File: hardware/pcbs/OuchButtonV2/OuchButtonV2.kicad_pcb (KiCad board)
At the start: 4 copper layers, 78 parts, among them J1 USB_C_Receptacle_USB2.0_14P, J3 Conn_01x01_Pin, Q1 AO3423 P-Chanel, U1 ESP32-C6-MINI-1/U, U2 RT9080-33GJ5, U3 MCP73831-2-OT, U4 MPU-6050, U5 DS1307Z+, U6 AT42QT1010-TSHR, U7 TS3A24159DGS, U8 AFE4404YZPT, U9 WE-TVS-82400102, Y1 32.768 kHz

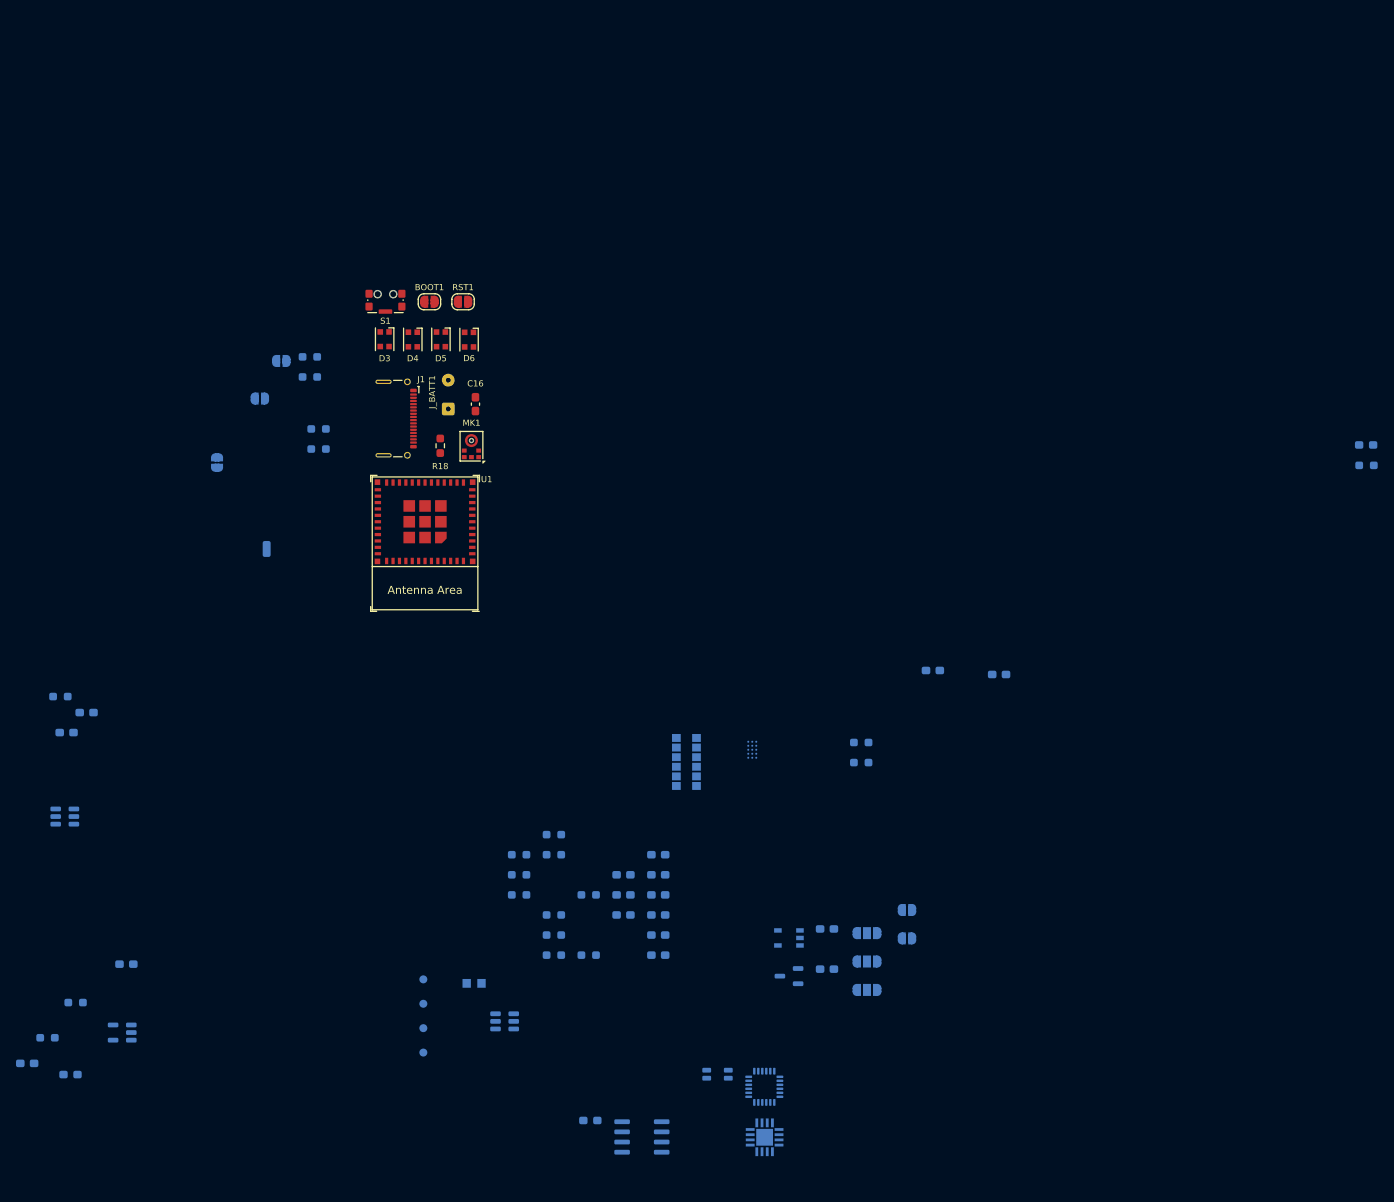
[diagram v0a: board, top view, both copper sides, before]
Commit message: Half done pcb
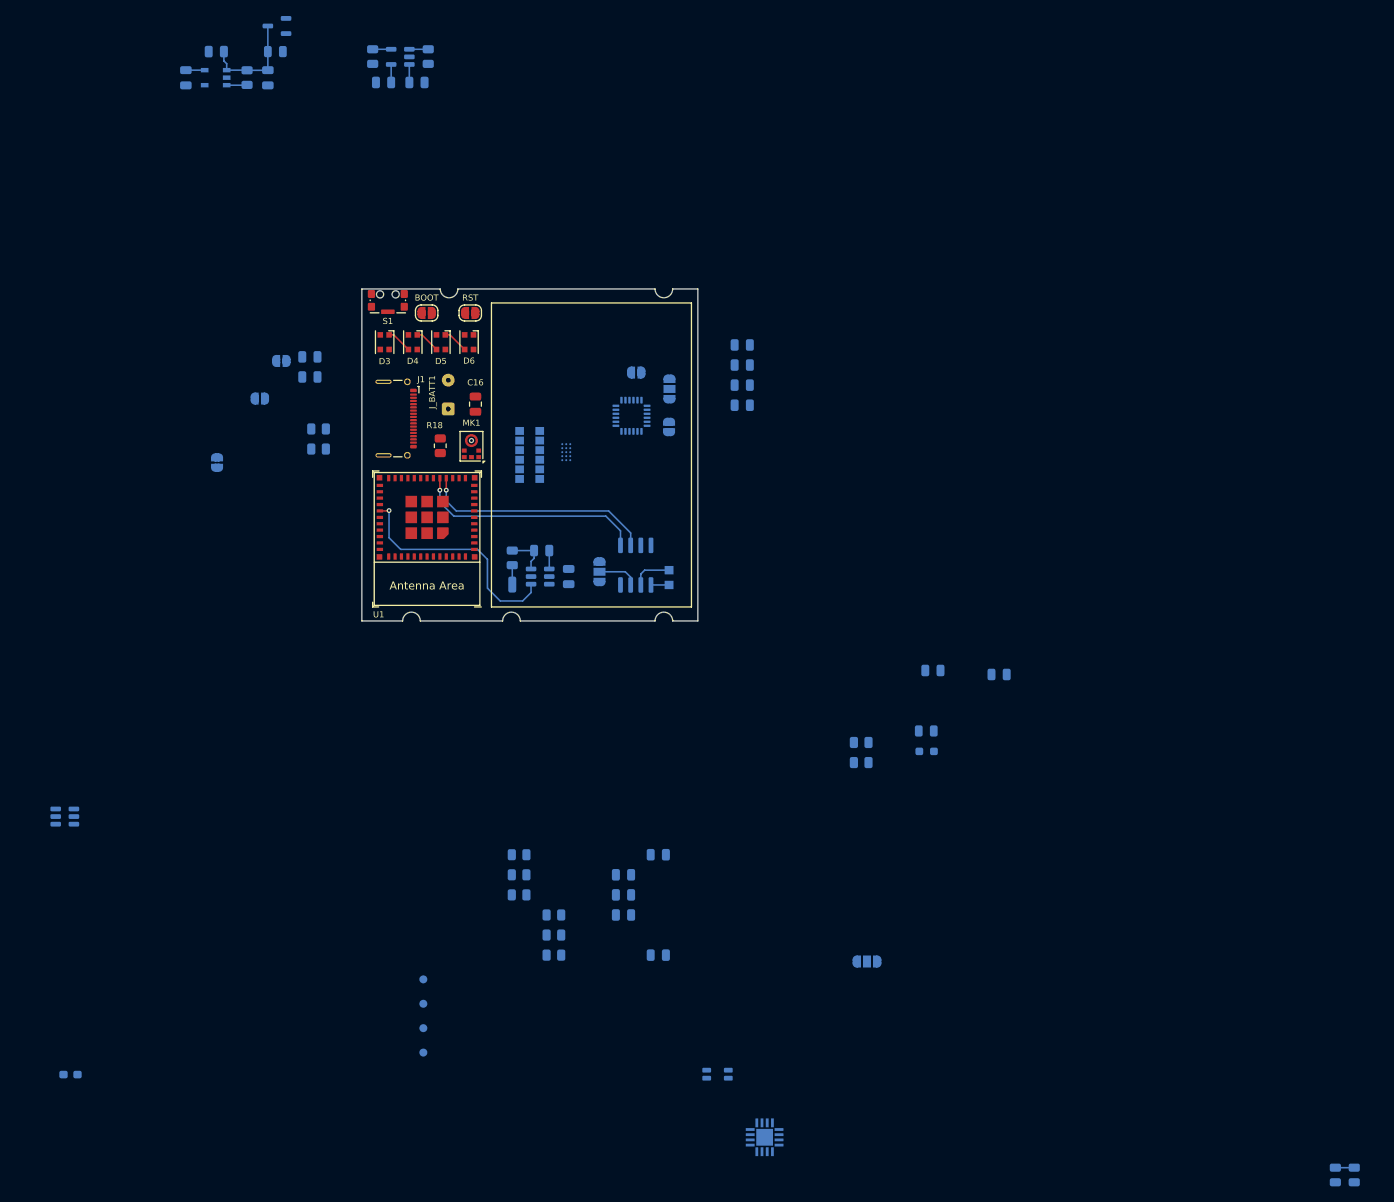
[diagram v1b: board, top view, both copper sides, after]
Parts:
- C1, C10, C11, C12, C13, C14, C15, C16, C17, C18, C2, C3, C4, C5, C6, C7, C8, C9: footprint Capacitor_SMD:C_0603_1608Metric_Pad1.08x0.95mm_HandSolder -> Capacitor_SMD:C_0805_2012Metric
- D1: footprint Diode_SMD:D_0603_1608Metric_Pad1.05x0.95mm_HandSolder -> Diode_SMD:D_0805_2012Metric
- D2: footprint LED_SMD:LED_0603_1608Metric_Pad1.05x0.95mm_HandSolder -> LED_SMD:LED_0805_2012Metric
- R1, R10, R11, R12, R13, R14, R15, R16, R17, R18, R2, R3, R4, R5, R6, R7, R9: footprint Resistor_SMD:R_0603_1608Metric_Pad0.98x0.95mm_HandSolder -> Resistor_SMD:R_0805_2012Metric
- R19, R20, R8: footprint Resistor_SMD:R_0603_1608Metric_Pad0.98x0.95mm_HandSolder -> Capacitor_SMD:C_0805_2012Metric
- moved D1 139.3 mm to (62.2, 41.3), turned to 0 degrees
- moved C5 137.8 mm to (54.8, 41.3)
- moved Q1 134.9 mm to (62.4, 38.1)
- moved C1 133.2 mm to (51.0, 44.6), turned to -90 degrees
- moved R4 131.6 mm to (81.3, 42.0), turned to 90 degrees
- moved C2 130.5 mm to (75.7, 45.2)
- moved U2 129.2 mm to (54.7, 44.6)
- moved U3 126.8 mm to (77.8, 42.0)
- moved R5 123.9 mm to (74.3, 42.0), turned to -90 degrees
- moved C3 116.0 mm to (79.9, 45.2), turned to 0 degrees
- moved R3 110.7 mm to (58.6, 44.6), turned to 90 degrees
- moved R7 108.7 mm to (197.1, 181.8), turned to 90 degrees
- moved R8 103.5 mm to (61.2, 44.6), turned to -90 degrees
- moved R6 97.3 mm to (194.7, 181.8), turned to -90 degrees
- moved U4 85.5 mm to (106.7, 86.8), turned to -90 degrees
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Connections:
- U1 pad 20: IO15/TOUCH -> unconnected-(U1-GPIO15-Pad20)
- U1 pad 29: IO23/AFE_RST -> IO23/TOUCH
- U6 pad 1: IO15/TOUCH -> IO23/TOUCH
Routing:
- net IO23/TOUCH: track 0.00 -> 29.2 mm, vias 0 -> 1
- net IO6/SDA: track 0.00 -> 29.1 mm, vias 0 -> 1
- net IO7/SCL: track 0.00 -> 28.9 mm, vias 0 -> 1
- net Net-(D1-K): track 0.00 -> 13.2 mm
- net Net-(U6-SNSK): track 0.00 -> 5.18 mm
- net Net-(JP8-C): track 0.00 -> 5.15 mm
- net Net-(U5-X2): track 0.00 -> 5.10 mm
- net Net-(D5-DOUT): track 0.00 -> 3.17 mm
- net Net-(D4-DOUT): track 0.00 -> 3.17 mm
- net Net-(D3-DOUT): track 0.00 -> 3.17 mm
- net Net-(U2-EN): track 0.00 -> 2.56 mm
- net Net-(J3-Pin_1): track 0.00 -> 2.42 mm
- net Net-(U6-SNS): track 0.00 -> 2.41 mm
- net IO2/BATT: track 0.00 -> 2.36 mm
- net IO3/CHG: track 0.00 -> 2.36 mm
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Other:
- board outline added: 42 x 41.5 mm
